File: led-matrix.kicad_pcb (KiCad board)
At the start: 2 copper layers, 103 x 52.5 mm, 138 parts

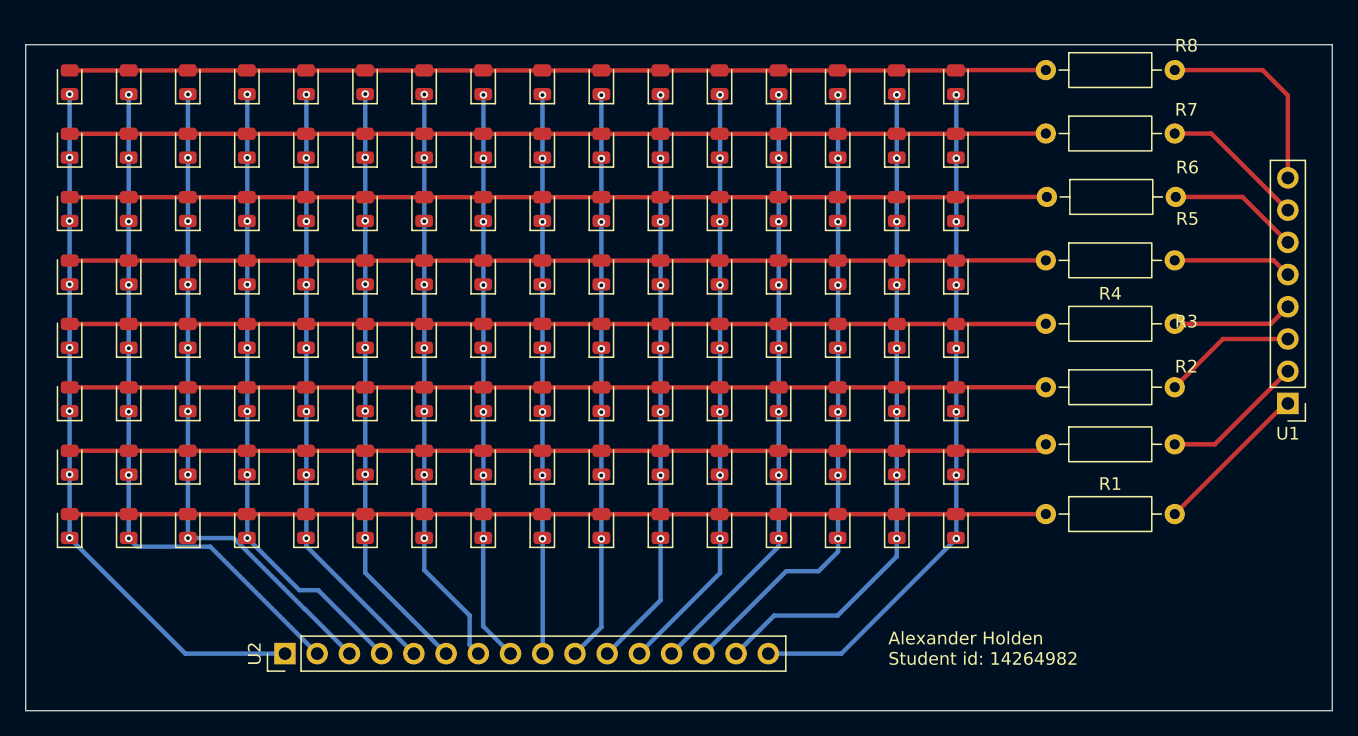
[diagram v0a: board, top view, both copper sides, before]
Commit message: made slight adjustments
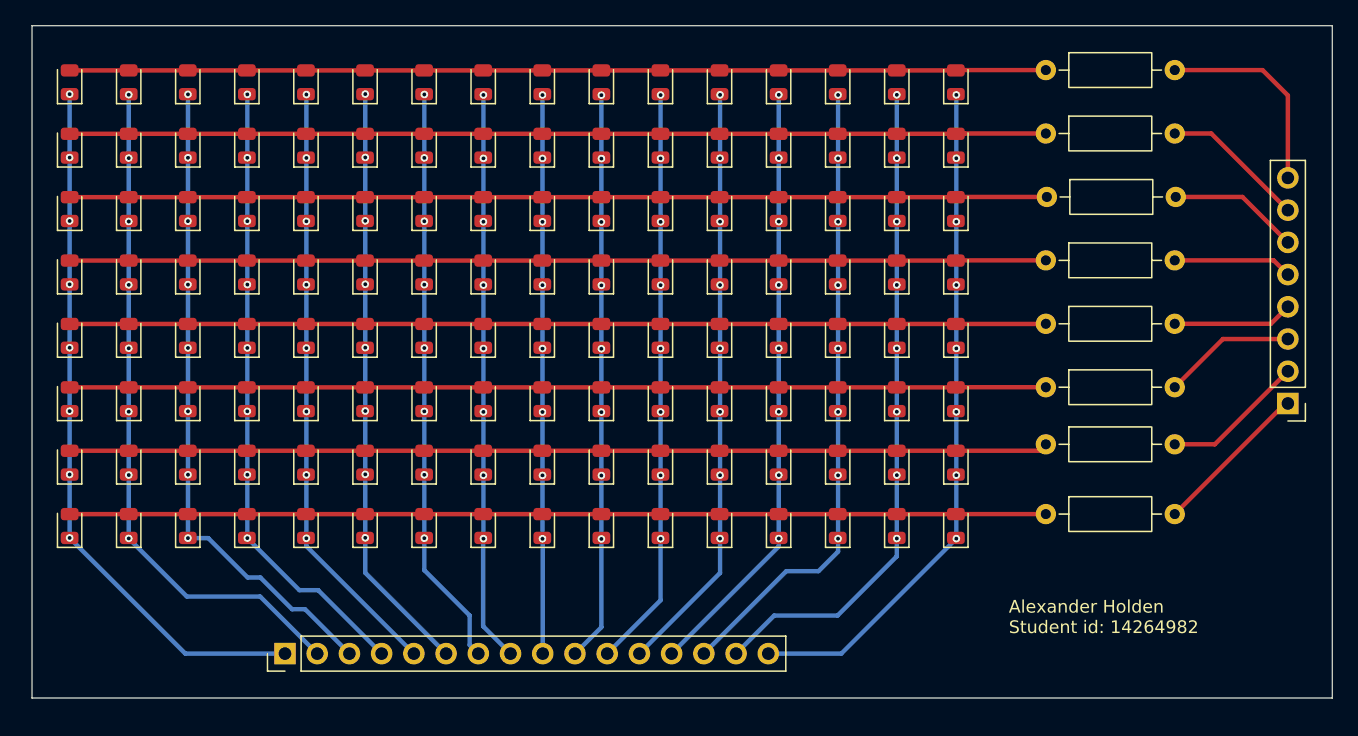
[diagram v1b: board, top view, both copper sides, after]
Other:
- board size 103 x 52.5 mm -> 102.5 x 53 mm
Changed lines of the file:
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@@
 		(tags "Resistor Axial_DIN0207 series Axial Horizontal pin pitch 10.16mm 0.25W = 1/4W length 6.3mm diameter 2.5mm")
 		(property "Reference" "R8"
-			(at 11.08 -1.92 0)
+			(at 5.08 -2.5 0)
 			(layer "F.SilkS")
+			(hide yes)
 			(effects
 				(font
@@
 			(at 11.08 -1.87 0)
 			(layer "F.SilkS")
+			(hide yes)
 			(effects
 				(font
@@
 			(at 11.16 -3.27 0)
 			(layer "F.SilkS")
+			(hide yes)
 			(effects
 				(font
@@
 			(at 11.08 -6.12 0)
 			(layer "F.SilkS")
+			(hide yes)
 			(effects
 				(font
@@
 			(at 0 -2.38 90)
 			(layer "F.SilkS")
+			(hide yes)
 			(effects
 				(font
@@
 			(at 11.08 -5.17 0)
 			(layer "F.SilkS")
+			(hide yes)
 			(effects
 				(font
@@
 			(at 5.08 -2.37 0)
 			(layer "F.SilkS")
+			(hide yes)
 			(effects
 				(font
@@
 			(at 5.08 -2.37 0)
 			(layer "F.SilkS")
+			(hide yes)
 			(effects
 				(font
@@
 			(at 11.08 -2.32 0)
 			(layer "F.SilkS")
+			(hide yes)
 			(effects
 				(font
@@
 			(at 0 2.5 0)
 			(layer "F.Fab")
+			(hide yes)
 			(effects
 				(font
@@
 			(at 0 -2.38 0)
 			(layer "F.SilkS")
+			(hide yes)
 			(effects
 				(font
@@
 	)
 	(gr_rect
-		(start 70 33)
-		(end 173 85.5)
+		(start 70.5 31.5)
+		(end 173 84.5)
 		(stroke
 			(width 0.05)
@@
 	)
 	(gr_text "Alexander Holden\nStudent id: 14264982"
-		(at 138 82 0)
+		(at 147.5 79.5 0)
 		(layer "F.SilkS")
 		(effects
@@
 	)
 	(segment
-		(start 84.550804 72.570804)
-		(end 78.775082 72.570804)
+		(start 88.48 76.5)
+		(end 92.98 81)
 		(width 0.35)
 		(layer "B.Cu")
@@
 	)
 	(segment
-		(start 92.98 81)
-		(end 84.550804 72.570804)
+		(start 78.124553 71.920275)
+		(end 82.704278 76.5)
 		(width 0.35)
 		(layer "B.Cu")
@@
 	)
 	(segment
-		(start 78.124553 71.920275)
-		(end 78.124553 36.941275)
+		(start 82.704278 76.5)
+		(end 88.48 76.5)
 		(width 0.35)
 		(layer "B.Cu")
@@
 	)
 	(segment
-		(start 78.775082 72.570804)
-		(end 78.124553 71.920275)
+		(start 78.124553 71.920275)
+		(end 78.124553 36.941275)
 		(width 0.35)
 		(layer "B.Cu")
@@
 	)
 	(segment
+		(start 88.5 75)
+		(end 91 77.5)
+		(width 0.35)
+		(layer "B.Cu")
+		(net 16)
+	)
+	(segment
 		(start 82.792157 71.894804)
-		(end 86.394804 71.894804)
+		(end 84.394804 71.894804)
+		(width 0.35)
+		(layer "B.Cu")
+		(net 16)
+	)
+	(segment
+		(start 84.394804 71.894804)
+		(end 87.5 75)
 		(width 0.35)
 		(layer "B.Cu")
@@
 	)
 	(segment
-		(start 92 77.5)
-		(end 92.02 77.5)
+		(start 87.5 75)
+		(end 88.5 75)
 		(width 0.35)
 		(layer "B.Cu")
@@
 	)
 	(segment
-		(start 86.394804 71.894804)
-		(end 92 77.5)
+		(start 91 77.5)
+		(end 92.02 77.5)
 		(width 0.35)
 		(layer "B.Cu")
